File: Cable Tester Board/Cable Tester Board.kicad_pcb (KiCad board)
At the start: 2 copper layers, 128 x 146 mm, 69 parts

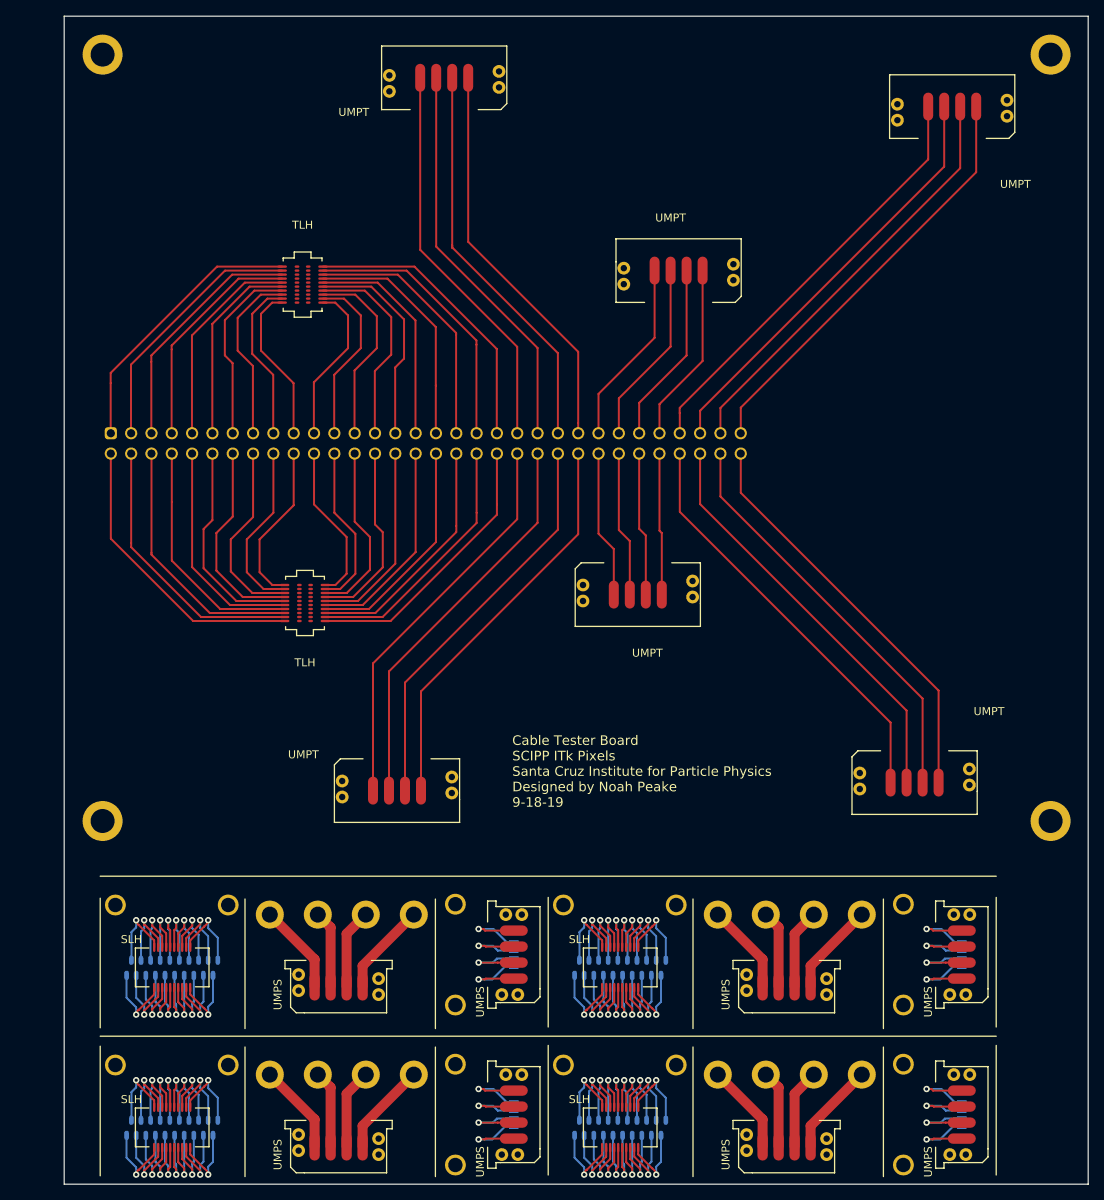
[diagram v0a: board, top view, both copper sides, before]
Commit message: Add files via upload
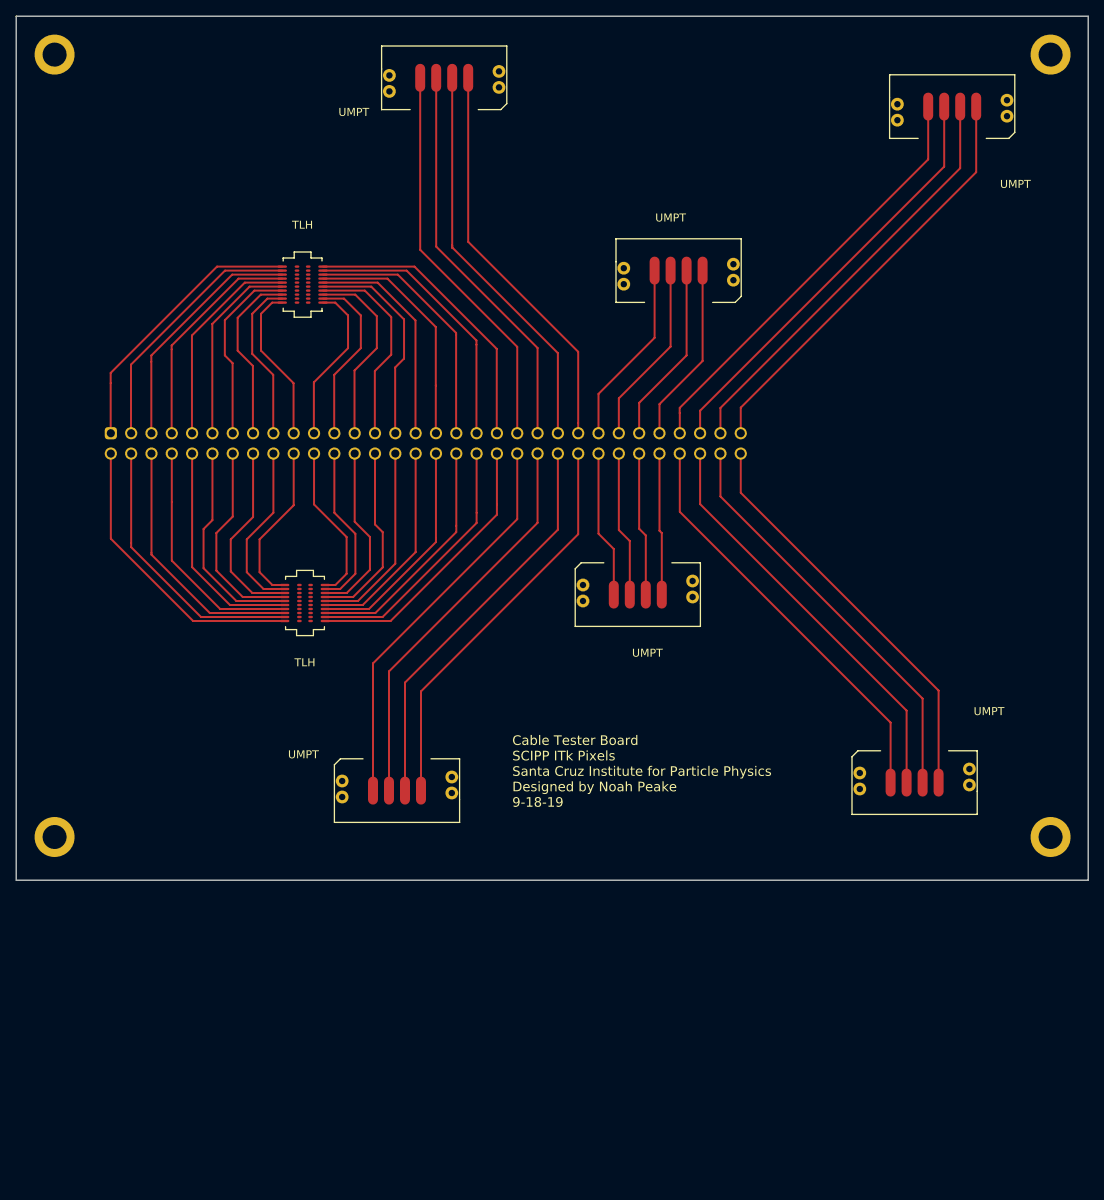
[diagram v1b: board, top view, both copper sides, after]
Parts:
- removed the REF** at (66.9, 166.2)
- removed the REF** at (35.6, 165.0)
- removed the REF** at (78.1, 177.5)
- removed the REF** at (72.9, 166.2)
- removed the REF** at (43.0, 171.9)
- removed the REF** at (78.1, 164.9)
- removed the REF** at (128.9, 166.2)
- removed the REF** at (99.0, 171.9)
- removed the REF** at (134.1, 164.9)
- removed the REF** at (134.1, 177.5)
- removed the REF** at (116.9, 166.2)
- removed the REF** at (85.4, 171.2) (x2)
- removed the REF** at (141.4, 171.2) (x2)
- removed the REF** at (110.9, 166.2)
- removed the REF** at (105.7, 165.0)
- removed the REF** at (122.9, 166.2)
- removed the REF** at (98.4, 173.8)
- removed the REF** at (98.7, 172.8)
- removed the REF** at (119.5, 175.2)
- removed the REF** at (91.6, 165.0)
- removed the REF** at (60.9, 166.2)
- removed the REF** at (122.9, 146.2)
- removed the REF** at (141.4, 151.2) (x2)
- removed the REF** at (116.9, 146.2)
- removed the REF** at (98.7, 152.8)
- removed the REF** at (105.7, 145.0)
- removed the REF** at (110.9, 146.2)
- removed the REF** at (42.7, 172.8)
- removed the REF** at (98.4, 153.8)
- removed the REF** at (119.5, 155.2)
- removed the REF** at (91.6, 145.0)
- removed the REF** at (134.1, 157.5)
- removed the REF** at (128.9, 146.2)
- removed the REF** at (99.0, 151.9)
- removed the REF** at (134.1, 144.9)
- removed the REF** at (63.5, 155.2)
- removed the REF** at (72.9, 146.2)
- removed the REF** at (49.7, 165.0)
- removed the REF** at (54.9, 146.2)
- removed the REF** at (66.9, 146.2)
- removed the REF** at (60.9, 146.2)
- removed the REF** at (49.7, 145.0)
- removed the REF** at (78.1, 144.9)
- removed the REF** at (42.4, 153.8)
- removed the REF** at (85.4, 151.2) (x2)
- removed the REF** at (35.6, 145.0)
- removed the REF** at (42.7, 152.8)
- removed the REF** at (54.9, 166.2)
- removed the REF** at (43.0, 151.9)
- removed the REF** at (78.1, 157.5)
- removed the REF** at (42.4, 173.8)
- removed the REF** at (63.5, 175.2)
- moved REF** 6.32 mm to (28.0, 136.5)
- moved REF** 6.00 mm to (28.0, 38.7)
- moved REF** 2.00 mm to (152.5, 136.5)
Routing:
- net (no net): track 3111.5 -> 2066.5 mm, vias 96 -> 0
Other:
- board size 128 x 146 mm -> 134 x 108 mm
- board text removed: "Type 1 Termination Board SCIPP ITk Pixels Designed by Noah Peake 9-18-19"
